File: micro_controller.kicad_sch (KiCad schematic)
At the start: 16 parts, among them J2 Conn_01x06_Male, Q7 DMN62D0U-7, U3 MCP2221A, U6 ESP32

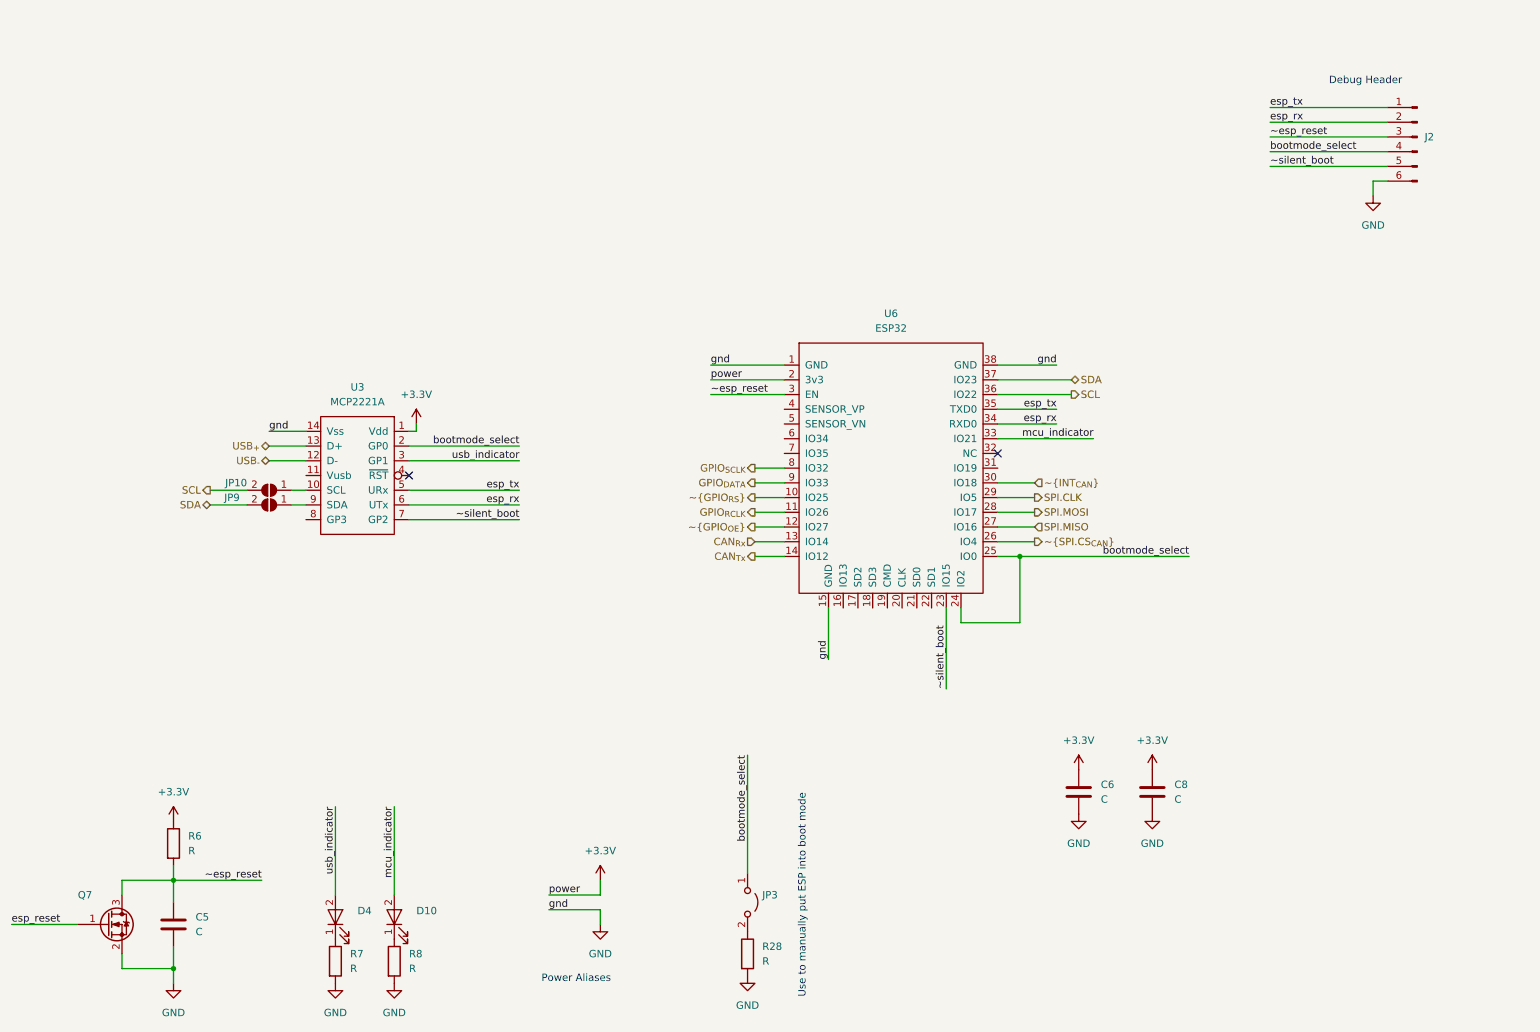
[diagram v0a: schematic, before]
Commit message: WIP
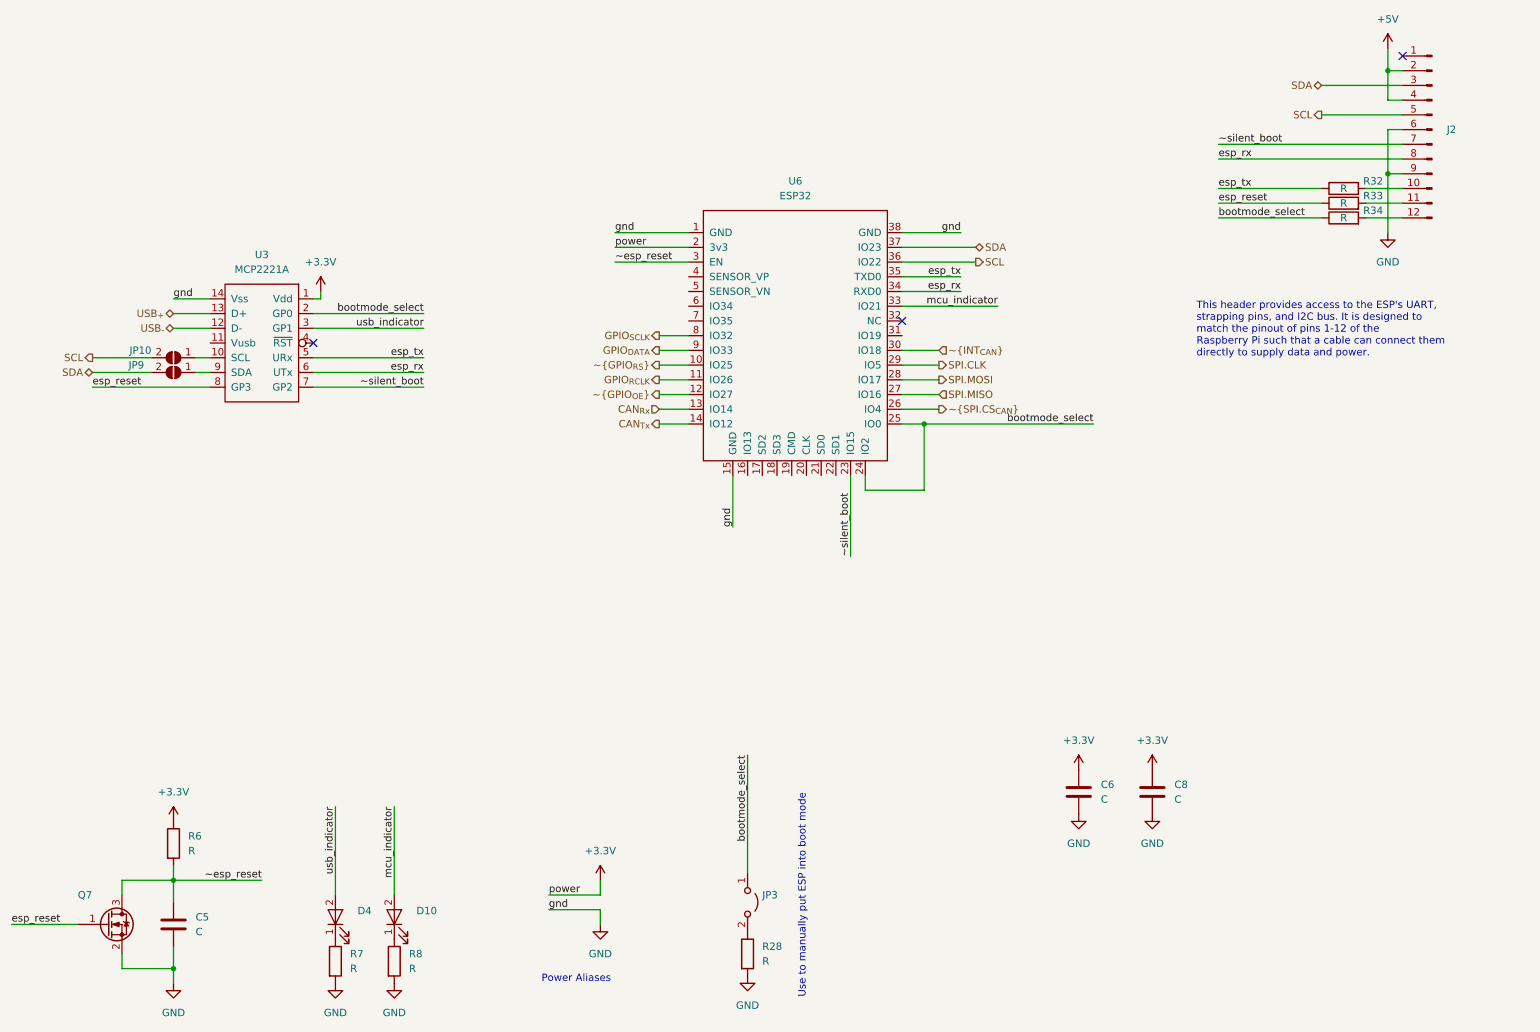
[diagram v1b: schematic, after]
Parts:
- removed J2: Conn_01x06_Male, Connector_PinHeader_2.54mm:PinHeader_2x03_P2.54mm_Vertical, symbol Connector:Conn_01x06_Male
- added J2: Conn_01x12_Male, Connector_PinHeader_2.54mm:PinHeader_2x06_P2.54mm_Vertical, symbol Connector:Conn_01x12_Male
- added R32, R33, R34: R, Resistor_SMD:R_0805_2012Metric, symbol Device:R
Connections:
- net GND: now also J2.6 (Pin_6), J2.9 (Pin_9)
- net SCL: now also J2.5 (Pin_5)
- net SDA: now also J2.3 (Pin_3)
- net bootmode_select: now also R34.1
- net esp_reset: now also U3.8 (GP3), R33.1
- net esp_rx: now also J2.8 (Pin_8)
- net esp_tx: now also R32.1
- net ~silent_boot: now also J2.7 (Pin_7)
- new net: J2.11 (Pin_11), R33.2
- new net: J2.10 (Pin_10), R32.2
- new net: J2.12 (Pin_12), R34.2
- new net +5V: J2.2 (Pin_2), J2.4 (Pin_4)
- no-connect marks 2 -> 3
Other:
- note added: "This header provides access to the ESP's UART, strapping pins, and I2C bus. It is designed to match the pinout of pins 1-12 of the Raspberry Pi such that a cable can connect them directly to supply data and power."
- note removed: "Debug Header"
- moved on the sheet: JP10, JP9, U3, U6
